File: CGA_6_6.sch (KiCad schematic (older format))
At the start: 8 parts, among them P5 Bus_ISA_8bit, U13 74LS08, U14 74LS32, U20 74LS04, U26 74S04, U41 74LS08, U42 74LS86, U66 74LS245

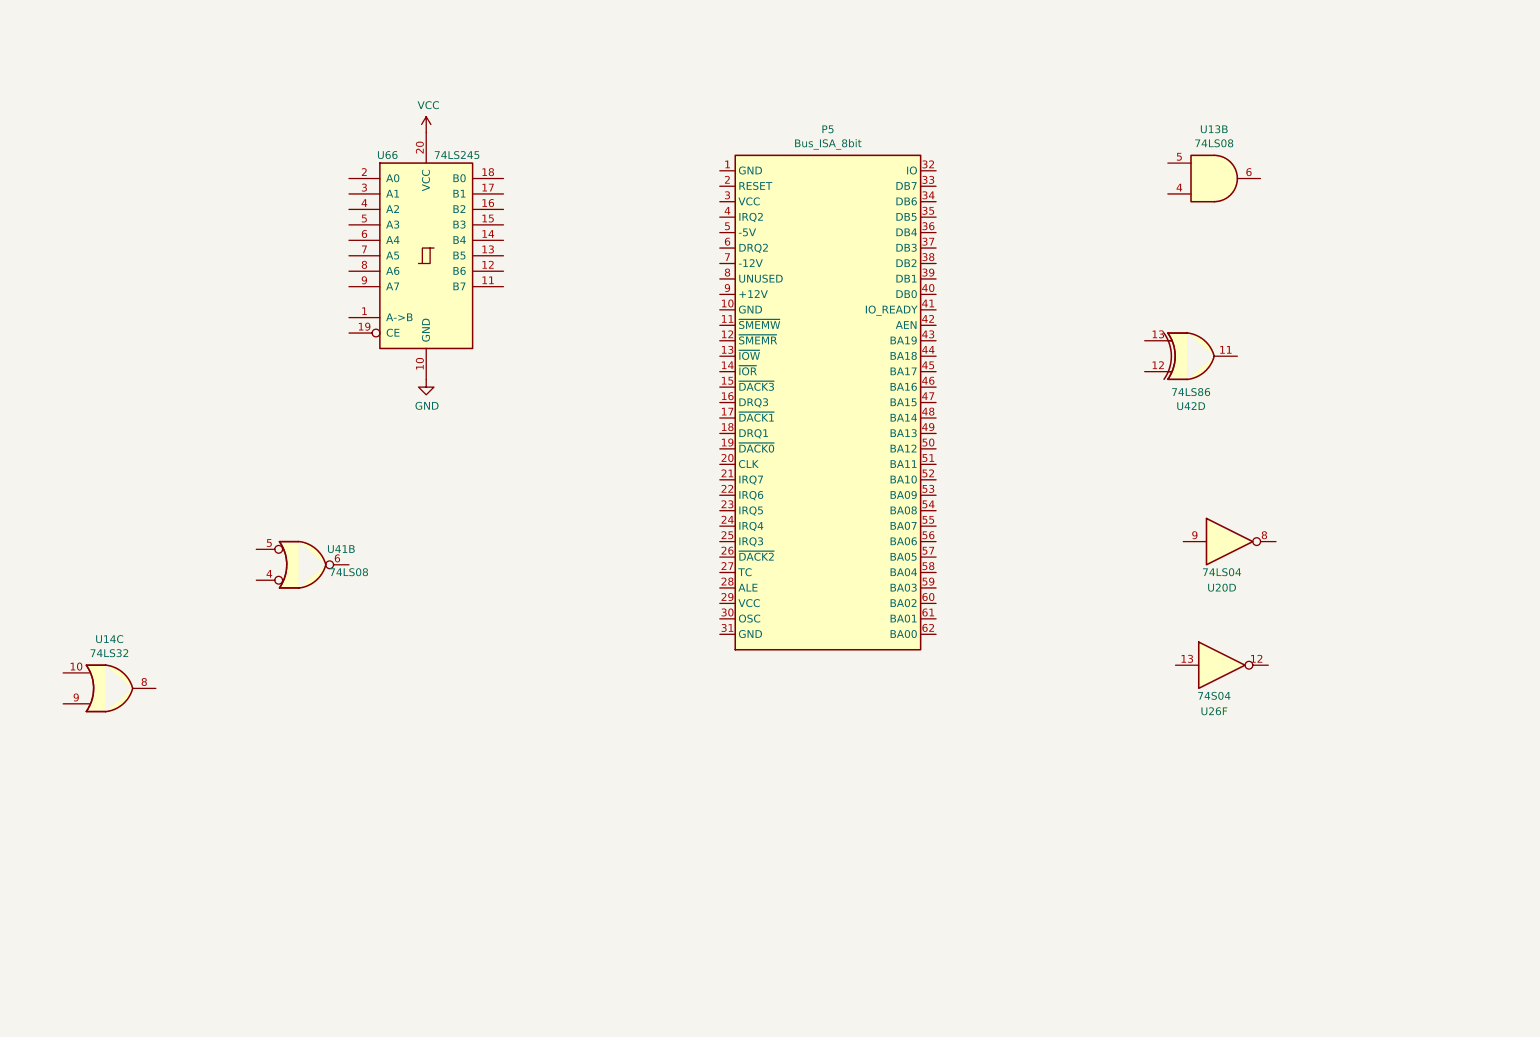
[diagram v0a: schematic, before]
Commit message: More sheet 6
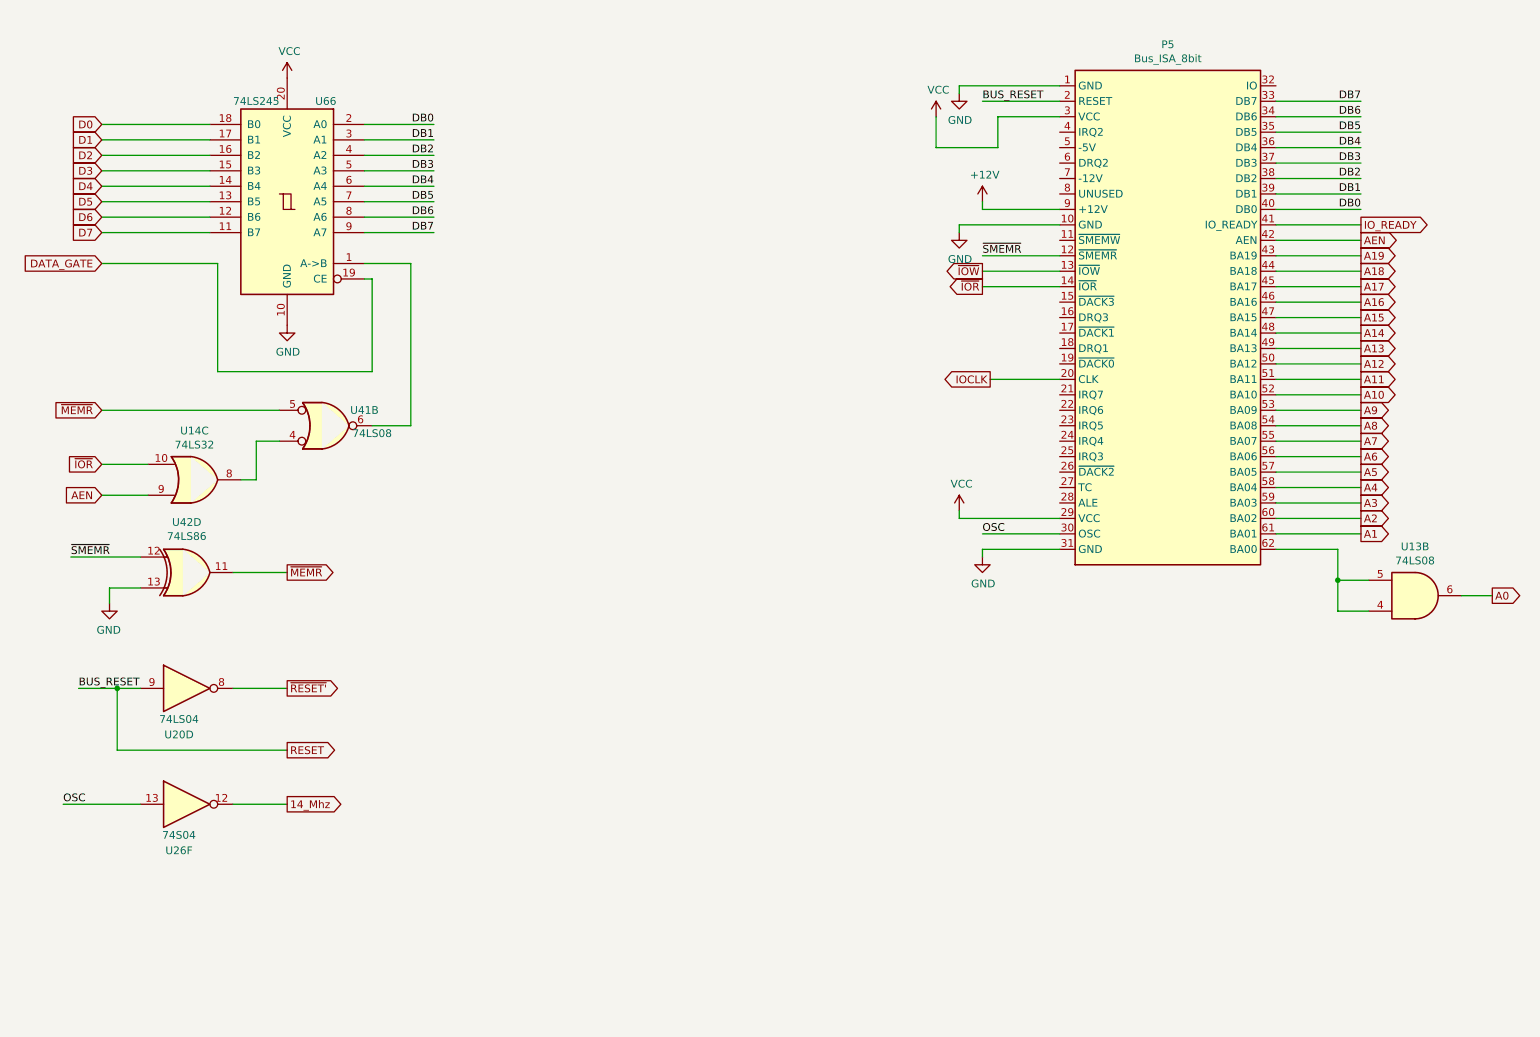
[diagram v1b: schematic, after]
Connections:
- net GND: now also P5.1 (GND), P5.10 (GND), P5.31 (GND), U42.13
- net VCC: now also P5.29 (VCC), P5.3 (VCC)
- net ~SMEMR: now reaches P5.12 (~SMEMR)
- net ~SMEMR: now also U42.12
- net ~IOW: now reaches P5.13 (~IOW)
- net ~IOR: now reaches P5.14 (~IOR)
- net ~IOR: now also U14.10
- net RESET: now reaches P5.2 (RESET)
- net RESET: now also U20.9
- net IOCLK: now reaches P5.20 (CLK)
- net OSC: now reaches P5.30 (OSC)
- net OSC: now also U26.13
- net DB7: now reaches P5.33 (DB7)
- net DB7: now also U66.9 (A7)
- net DB6: now reaches P5.34 (DB6)
- net DB6: now also U66.8 (A6)
- net DB5: now reaches P5.35 (DB5)
- net DB5: now also U66.7 (A5)
- net DB4: now reaches P5.36 (DB4)
- net DB4: now also U66.6 (A4)
- net DB3: now reaches P5.37 (DB3)
- net DB3: now also U66.5 (A3)
- net DB2: now reaches P5.38 (DB2)
- net DB2: now also U66.4 (A2)
- net DB1: now reaches P5.39 (DB1)
- net DB1: now also U66.3 (A1)
- net DB0: now reaches P5.40 (DB0)
- net DB0: now also U66.2 (A0)
- net IO_READY: now reaches P5.41 (IO_READY)
- net AEN: now reaches P5.42 (AEN)
- net AEN: now also U14.9
- net A19: now reaches P5.43 (BA19)
- net A18: now reaches P5.44 (BA18)
- net A17: now reaches P5.45 (BA17)
- net A16: now reaches P5.46 (BA16)
- net A15: now reaches P5.47 (BA15)
- net A14: now reaches P5.48 (BA14)
- net A13: now reaches P5.49 (BA13)
- net A12: now reaches P5.50 (BA12)
- net A11: now reaches P5.51 (BA11)
- net A10: now reaches P5.52 (BA10)
- net A9: now reaches P5.53 (BA09)
- net A8: now reaches P5.54 (BA08)
- net A7: now reaches P5.55 (BA07)
- net A6: now reaches P5.56 (BA06)
- net A5: now reaches P5.57 (BA05)
- net A4: now reaches P5.58 (BA04)
- net A3: now reaches P5.59 (BA03)
- net A2: now reaches P5.60 (BA02)
- net A1: now reaches P5.61 (BA01)
- net at P5.62 (BA00): now also U13.4, U13.5
- net +12V: now reaches P5.9 (+12V)
- net at U66.1 (A->B): now also U41.6
- net D7: now reaches U66.11 (B7)
- net D6: now reaches U66.12 (B6)
- net D5: now reaches U66.13 (B5)
- net D4: now reaches U66.14 (B4)
- net D3: now reaches U66.15 (B3)
- net D2: now reaches U66.16 (B2)
- net D1: now reaches U66.17 (B1)
- net D0: now reaches U66.18 (B0)
- net DATA_GATE: now reaches U66.19 (CE)
- net at U41.4: now also U14.8
- net ~MEMR: now reaches U41.5
- net ~MEMR: now also U42.11
- net A0: now reaches U13.6
- net ~RESET': now reaches U20.8
- net 14_Mhz: now reaches U26.12
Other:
- moved on the sheet: P5, U13B, U14C, U20D, U26F, U41B, U66

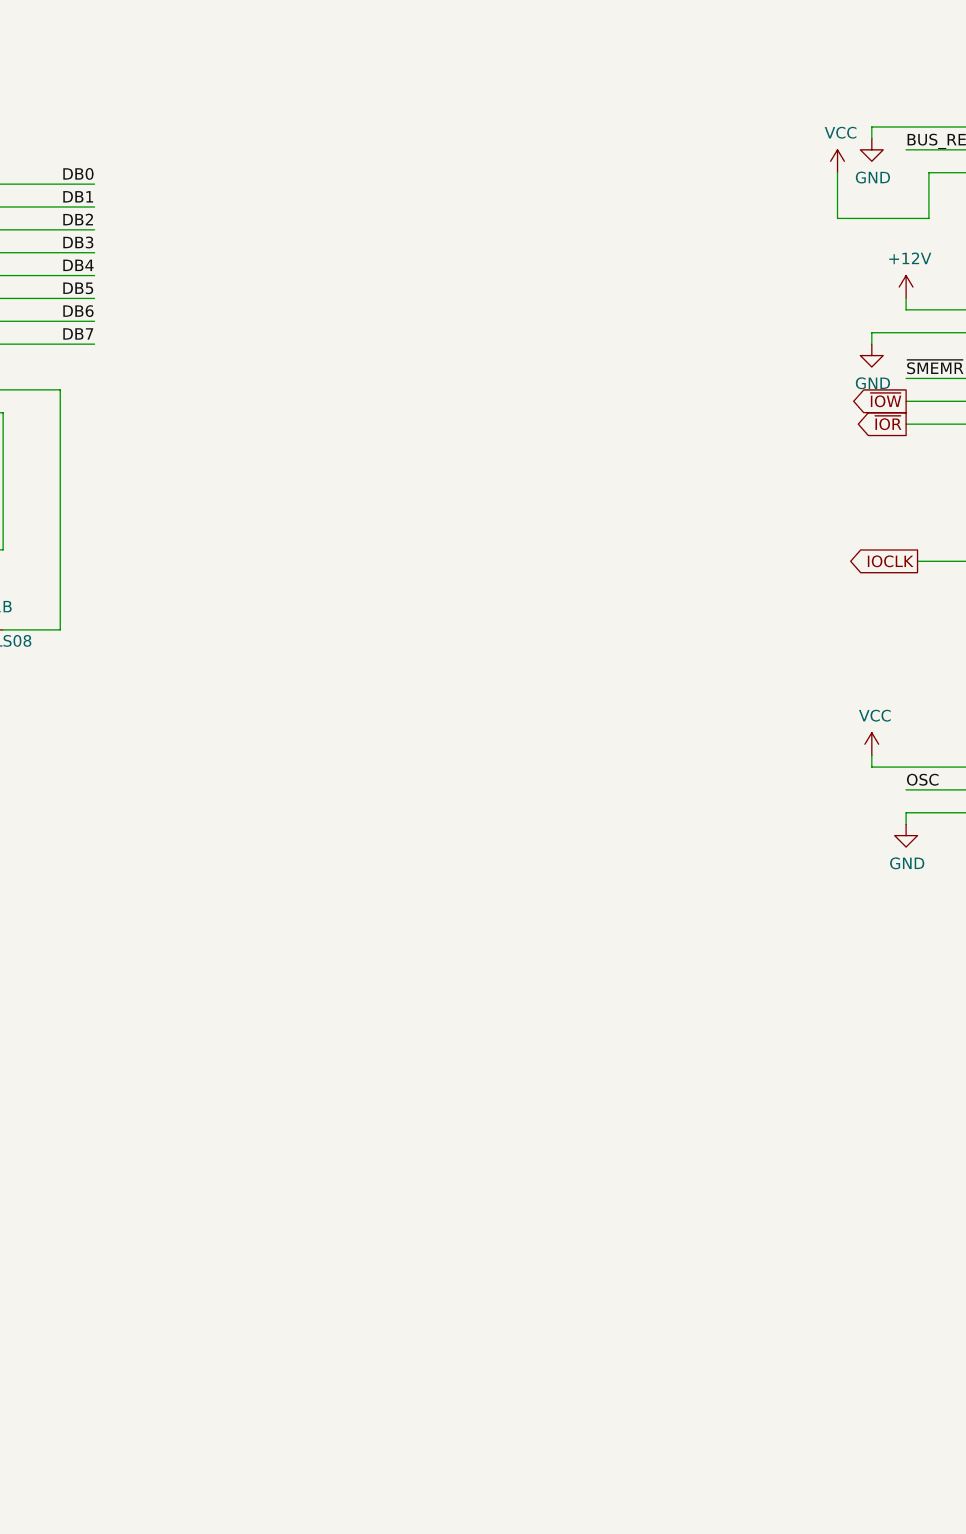
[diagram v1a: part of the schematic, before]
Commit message: Sheet 6
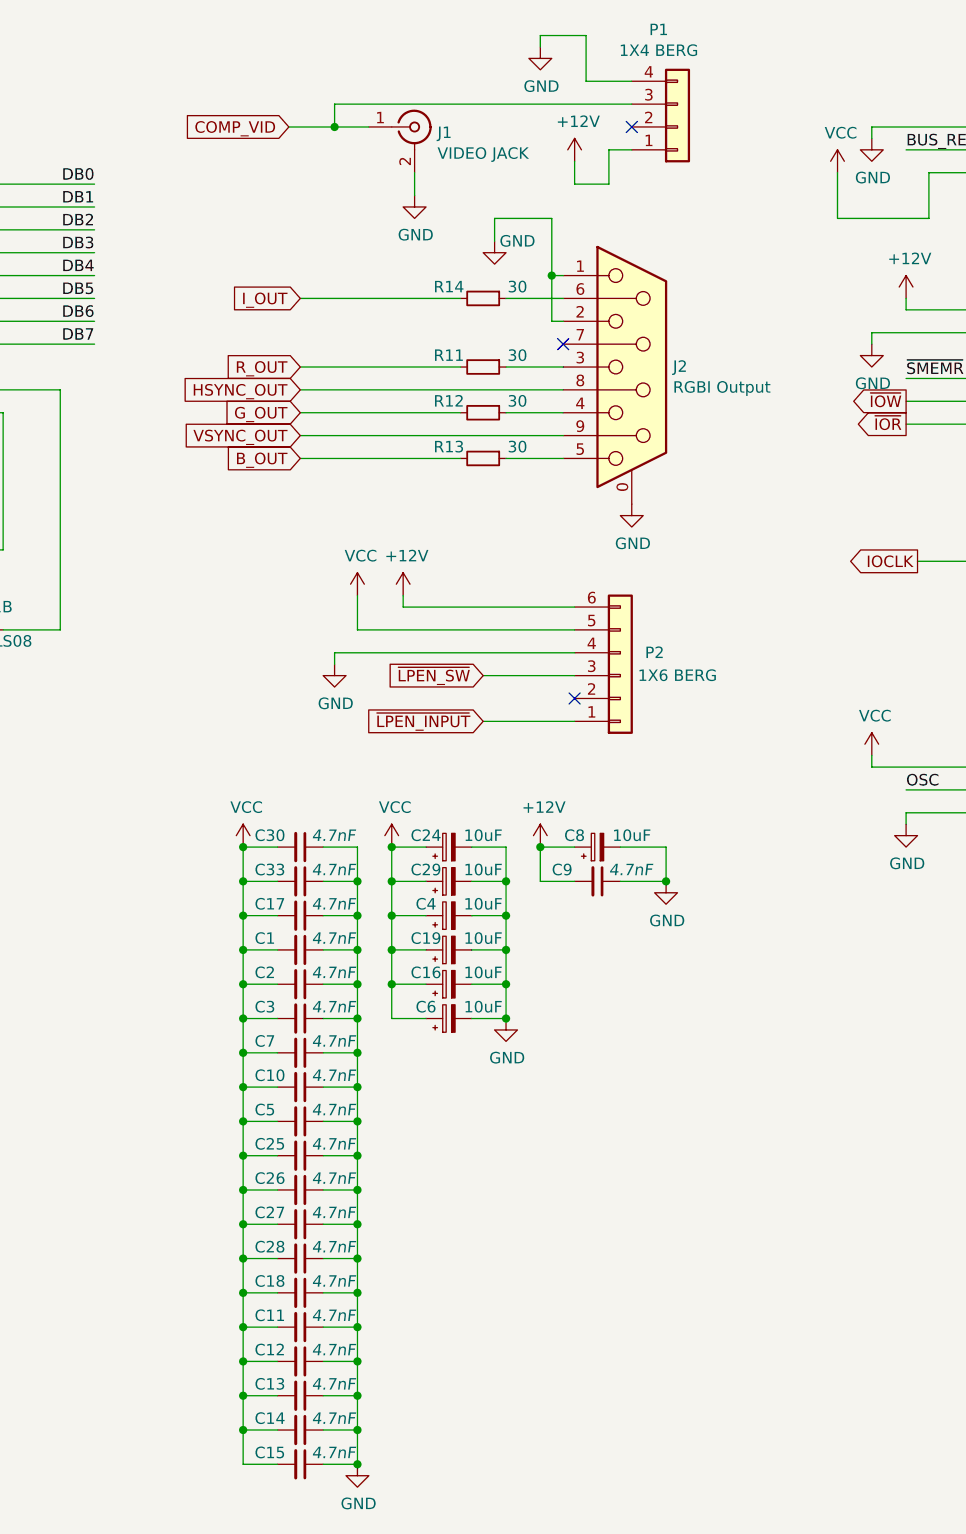
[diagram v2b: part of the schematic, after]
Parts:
- added C1, C10, C11, C12, C13, C14, C15, C17, C18, C2, C25, C26, C27, C28, C3, C30, C33, C5, C7, C9: 4.7nF, Capacitor_THT:C_Disc_D4.3mm_W1.9mm_P5.00mm, symbol Device:C_Small
- added C16, C19, C24, C29, C4, C6, C8: 10uF, Capacitor_THT:CP_Radial_D8.0mm_P5.00mm, symbol Device:CP_Small
- added J1: VIDEO JACK, symbol Connector:Conn_Coaxial
- added J2: RGBI Output, symbol Connector:DB9_Female_MountingHoles
- added P1: 1X4 BERG, symbol Connector_Generic:Conn_01x04
- added P2: 1X6 BERG, symbol Connector_Generic:Conn_01x06
- added R11, R12, R13, R14: 30, Resistor_THT:R_Axial_DIN0207_L6.3mm_D2.5mm_P10.16mm_Horizontal, symbol Device:R_Small
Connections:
- net +12V: now also C8.1, C9.2, P1.1 (Pin_1), P2.6 (Pin_6)
- net GND: now also C1.1, C10.1, C11.1, C12.1, C13.1, C14.1, C15.1, C16.2, C17.1, C18.1, C19.2, C2.1, C24.2, C25.1, C26.1, C27.1, C28.1, C29.2, C3.1, C30.1, C33.1, C4.2, C5.1, C6.2, C7.1, C8.2, C9.1, J1.2 (Ext), J2.0 (PAD), J2.1, J2.2, P1.4 (Pin_4), P2.4 (Pin_4)
- net VCC: now also C1.2, C10.2, C11.2, C12.2, C13.2, C14.2, C15.2, C16.1, C17.2, C18.2, C19.1, C2.2, C24.1, C25.2, C26.2, C27.2, C28.2, C29.1, C3.2, C30.2, C33.2, C4.1, C5.2, C6.1, C7.2, P2.5 (Pin_5)
- new net: J2.6, R14.1
- new net: J2.3, R11.1
- new net: J2.4, R12.1
- new net: J2.5, R13.1
- new net B_OUT: R13.2
- new net COMP_VID: J1.1 (In), P1.3 (Pin_3)
- new net G_OUT: R12.2
- new net HSYNC_OUT: J2.8
- new net I_OUT: R14.2
- new net R_OUT: R11.2
- new net VSYNC_OUT: J2.9
- new net ~LPEN_INPUT: P2.1 (Pin_1)
- new net ~LPEN_SW: P2.3 (Pin_3)
- no-connect marks 0 -> 3
